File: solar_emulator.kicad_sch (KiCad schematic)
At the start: 80 parts, among them J1 USB_C_Receptacle_USB2.0_16P, J2 Conn_01x02, J3 Conn_01x02, J4 Conn_01x02, J5 Conn_01x02, J6 Conn_01x03, J7 Conn_01x04, Q1 IRFZ44N, Q2 IRFZ44N, Q3 IRFZ44N, Q4 IRFZ44N, Q5 IRFZ44N, Q6 IRFZ44N, Q7 IRFZ44N, Q8 IRFZ44N, SW1 SW_Push, SW2 SW_Push, U1 ESP32-S3-WROOM-1, U2 LD1117S33TR_SOT223, U3 HIP4081AIPZ, U4 HIP4081AIPZ, U5 LM393, U6 LM393, U7 USBLC6-2SC6

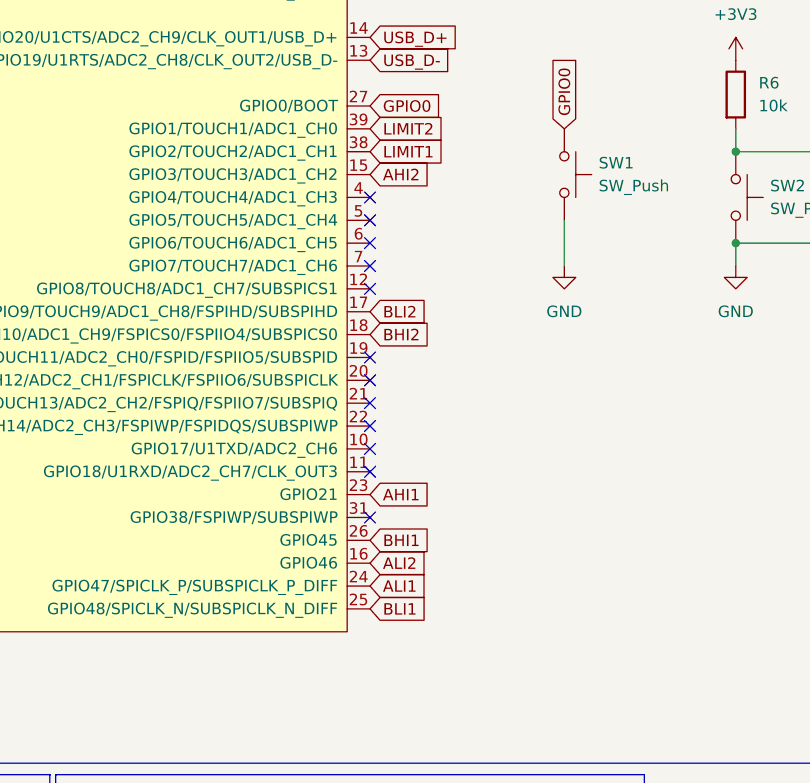
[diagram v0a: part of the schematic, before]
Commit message: tracing complete, need to optimize pcb
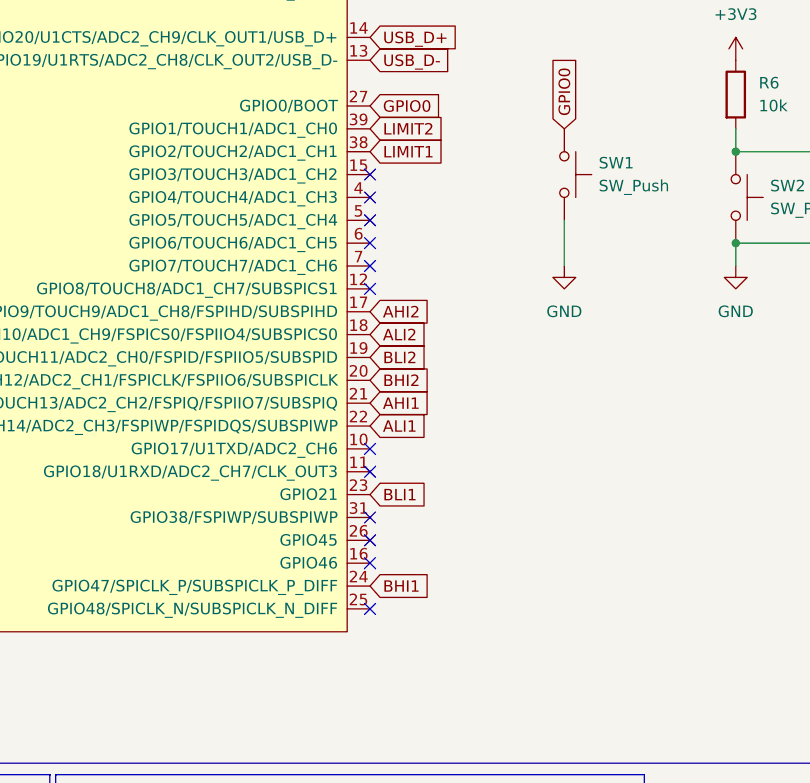
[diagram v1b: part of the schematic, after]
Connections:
- net AHI1: now also U1.21 (GPIO13/TOUCH13/ADC2_CH2/FSPIQ/FSPIIO7/SUBSPIQ); no longer U1.23 (GPIO21)
- net AHI2: now also U1.17 (GPIO9/TOUCH9/ADC1_CH8/FSPIHD/SUBSPIHD); no longer U1.15 (GPIO3/TOUCH3/ADC1_CH2)
- net ALI1: now also U1.22 (GPIO14/TOUCH14/ADC2_CH3/FSPIWP/FSPIDQS/SUBSPIWP); no longer U1.24 (GPIO47/SPICLK_P/SUBSPICLK_P_DIFF)
- net ALI2: now also U1.18 (GPIO10/TOUCH10/ADC1_CH9/FSPICS0/FSPIIO4/SUBSPICS0); no longer U1.16 (GPIO46)
- net BHI1: now also U1.24 (GPIO47/SPICLK_P/SUBSPICLK_P_DIFF); no longer U1.26 (GPIO45)
- net BHI2: now also U1.20 (GPIO12/TOUCH12/ADC2_CH1/FSPICLK/FSPIIO6/SUBSPICLK); no longer U1.18 (GPIO10/TOUCH10/ADC1_CH9/FSPICS0/FSPIIO4/SUBSPICS0)
- net BLI1: now also U1.23 (GPIO21); no longer U1.25 (GPIO48/SPICLK_N/SUBSPICLK_N_DIFF)
- net BLI2: now also U1.19 (GPIO11/TOUCH11/ADC2_CH0/FSPID/FSPIIO5/SUBSPID); no longer U1.17 (GPIO9/TOUCH9/ADC1_CH8/FSPIHD/SUBSPIHD)
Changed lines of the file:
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@@
 	)
 	(no_connect
-		(at 118.11 69.85)
+		(at 118.11 49.53)
 	)
 	(no_connect
@@
 	)
 	(no_connect
-		(at 118.11 77.47)
+		(at 118.11 90.17)
 	)
 	(no_connect
@@
 	)
 	(no_connect
-		(at 118.11 74.93)
+		(at 118.11 97.79)
 	)
 	(no_connect
-		(at 118.11 72.39)
+		(at 118.11 92.71)
 	)
 	(no_connect
@@
 	(global_label "BHI2"
 		(shape input)
-		(at 118.11 67.31 0)
+		(at 118.11 72.39 0)
 		(fields_autoplaced yes)
 		(effects
@@
 		)
 		(property "Intersheetrefs" "${INTERSHEET_REFS}"
-			(at 125.51 67.31 0)
+			(at 125.51 72.39 0)
 			(hide yes)
 			(show_name no)
@@
 	(global_label "ALI2"
 		(shape input)
-		(at 118.11 92.71 0)
+		(at 118.11 67.31 0)
 		(fields_autoplaced yes)
 		(effects
@@
 		)
 		(property "Intersheetrefs" "${INTERSHEET_REFS}"
-			(at 125.0262 92.71 0)
+			(at 125.0262 67.31 0)
 			(hide yes)
 			(show_name no)
@@
 	(global_label "BLI2"
 		(shape input)
-		(at 118.11 64.77 0)
+		(at 118.11 69.85 0)
 		(fields_autoplaced yes)
 		(effects
@@
 		)
 		(property "Intersheetrefs" "${INTERSHEET_REFS}"
-			(at 125.2076 64.77 0)
+			(at 125.2076 69.85 0)
 			(hide yes)
 			(show_name no)
@@
 	(global_label "BLI1"
 		(shape input)
-		(at 118.11 97.79 0)
+		(at 118.11 85.09 0)
 		(fields_autoplaced yes)
 		(effects
@@
 		)
 		(property "Intersheetrefs" "${INTERSHEET_REFS}"
-			(at 126.9614 97.79 0)
+			(at 126.9614 85.09 0)
 			(hide yes)
 			(show_name no)
@@
 	(global_label "AHI2"
 		(shape input)
-		(at 118.11 49.53 0)
+		(at 118.11 64.77 0)
 		(fields_autoplaced yes)
 		(effects
@@
 		)
 		(property "Intersheetrefs" "${INTERSHEET_REFS}"
-			(at 125.3286 49.53 0)
+			(at 125.3286 64.77 0)
 			(hide yes)
 			(show_name no)
@@
 	(global_label "AHI1"
 		(shape input)
-		(at 118.11 85.09 0)
+		(at 118.11 74.93 0)
 		(fields_autoplaced yes)
 		(effects
@@
 		)
 		(property "Intersheetrefs" "${INTERSHEET_REFS}"
-			(at 125.3286 85.09 0)
+			(at 125.3286 74.93 0)
 			(hide yes)
 			(show_name no)
@@
 	(global_label "ALI1"
 		(shape input)
-		(at 118.11 95.25 0)
+		(at 118.11 77.47 0)
 		(fields_autoplaced yes)
 		(effects
@@
 		)
 		(property "Intersheetrefs" "${INTERSHEET_REFS}"
-			(at 125.0262 95.25 0)
+			(at 125.0262 77.47 0)
 			(hide yes)
 			(show_name no)
@@
 	(global_label "BHI1"
 		(shape input)
-		(at 118.11 90.17 0)
+		(at 118.11 95.25 0)
 		(fields_autoplaced yes)
 		(effects
@@
 		)
 		(property "Intersheetrefs" "${INTERSHEET_REFS}"
-			(at 126.9614 90.17 0)
+			(at 126.9614 95.25 0)
 			(hide yes)
 			(show_name no)
